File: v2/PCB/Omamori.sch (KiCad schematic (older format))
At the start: 28 parts, among them J1 Conn_01x04_Female, U1 BQ25504, U2 TPS61222DCK, U3 ATtiny85, U4 TS-1233

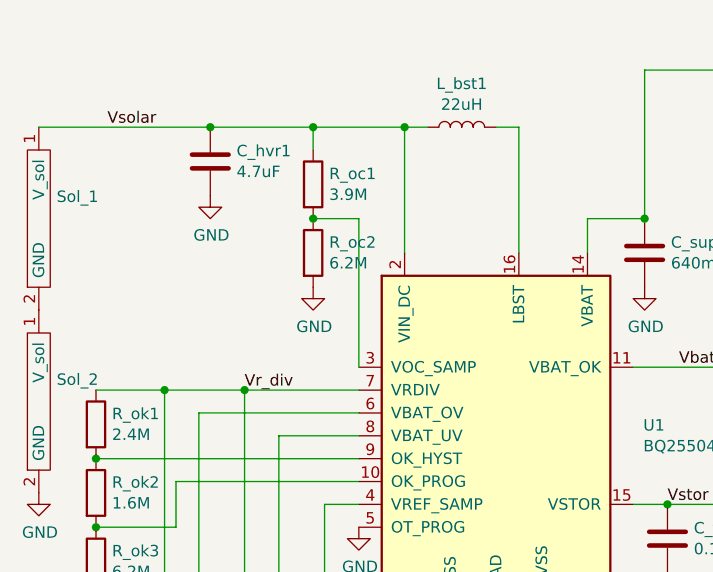
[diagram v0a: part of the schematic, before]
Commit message: Beyond last second changes to the PCB design and gerber files.
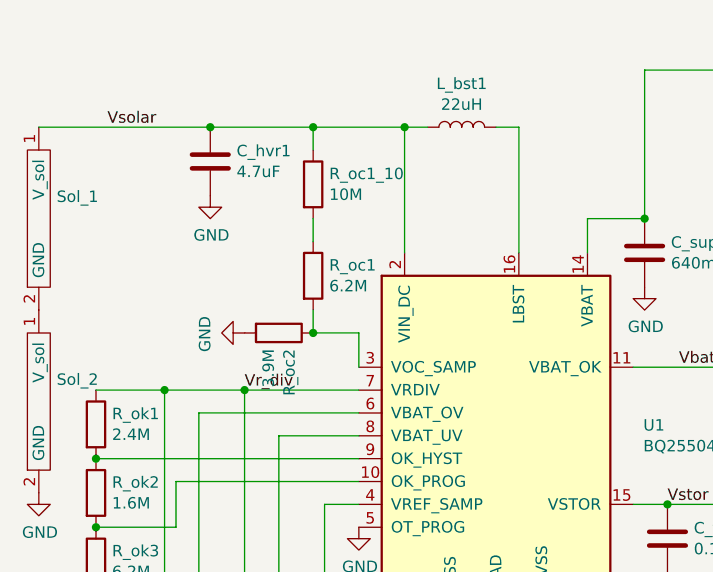
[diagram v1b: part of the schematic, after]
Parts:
- added R_oc1: 6.2M, Resistor_SMD:R_0603_1608Metric_Pad0.98x0.95mm_HandSolder, symbol Device:R
- R_oc1_10: renamed from R_oc1; value 3.9M -> 10M
- R_oc2: value 6.2M -> 3.9M
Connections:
- net at R_oc2.1, U1.3 (VOC_SAMP): now also R_oc1.2; no longer R_oc1_10.2
- new net: R_oc1.1, R_oc1_10.2
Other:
- moved on the sheet: R_oc2
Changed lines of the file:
@@
-$EndComp
-$Comp
-L Battery_Management:BQ25504 U1
-U 1 1 6049F0BD
-P 4550 3400
-F 0 "U1" H 5194 3446 50  0000 L CNN
-F 1 "BQ25504" H 5194 3355 50  0000 L CNN
-F 2 "footprints:VQFN-16-1EP_3x3mm_P0.5mm_EP1.8x1.8mm" H 4550 3400 50  0001 C CNN
-F 3 "http://www.ti.com/lit/ds/symlink/bq25504.pdf" H 4250 4200 50  0001 C CNN
-	1    4550 3400
-	1    0    0    -1
 $EndComp
 $Comp
@@
 Connection ~ 4150 2050
 $Comp
-L Device:R R_oc1
+L Device:R R_oc1_10
 U 1 1 609D50F7
 P 3750 2300
-F 0 "R_oc1" H 3820 2346 50  0000 L CNN
-F 1 "3.9M" H 3820 2255 50  0000 L CNN
+F 0 "R_oc1_10" H 3820 2346 50  0000 L CNN
+F 1 "10M" H 3820 2255 50  0000 L CNN
 F 2 "Resistor_SMD:R_0603_1608Metric_Pad1.05x0.95mm_HandSolder" V 3680 2300 50  0001 C CNN
 F 3 "~" H 3750 2300 50  0001 C CNN
@@
 L Device:R R_oc2
 U 1 1 609D577E
-P 3750 2600
-F 0 "R_oc2" H 3820 2646 50  0000 L CNN
-F 1 "6.2M" H 3820 2555 50  0000 L CNN
-F 2 "Resistor_SMD:R_0603_1608Metric_Pad1.05x0.95mm_HandSolder" V 3680 2600 50  0001 C CNN
-F 3 "~" H 3750 2600 50  0001 C CNN
-	1    3750 2600
-	1    0    0    -1
+P 3600 2950
+F 0 "R_oc2" H 3670 2996 50  0000 L CNN
+F 1 "3.9M" H 3670 2905 50  0000 L CNN
+F 2 "Resistor_SMD:R_0603_1608Metric_Pad1.05x0.95mm_HandSolder" V 3530 2950 50  0001 C CNN
+F 3 "~" H 3600 2950 50  0001 C CNN
+	1    3600 2950
+	0    1    1    0
 $EndComp
 Wire Wire Line
@@
 Wire Wire Line
 	3750 2050 4150 2050
-Wire Wire Line
-	3750 2450 3950 2450
-Wire Wire Line
-	3950 2450 3950 3100
-Connection ~ 3750 2450
 $Comp
 L power:GND #PWR06
 U 1 1 609DECA8
-P 3750 2750
-F 0 "#PWR06" H 3750 2500 50  0001 C CNN
-F 1 "GND" H 3755 2577 50  0000 C CNN
-F 2 "" H 3750 2750 50  0001 C CNN
-F 3 "" H 3750 2750 50  0001 C CNN
-	1    3750 2750
-	1    0    0    -1
+P 3450 2950
+F 0 "#PWR06" H 3450 2700 50  0001 C CNN
+F 1 "GND" H 3455 2777 50  0000 C CNN
+F 2 "" H 3450 2950 50  0001 C CNN
+F 3 "" H 3450 2950 50  0001 C CNN
+	1    3450 2950
+	0    1    1    0
 $EndComp
 Wire Wire Line
@@
 	5200 1800 5200 2450
 Connection ~ 5200 2450
+$Comp
+L Battery_Management:BQ25504 U1
+U 1 1 6049F0BD
+P 4550 3400
+F 0 "U1" H 5194 3446 50  0000 L CNN
+F 1 "BQ25504" H 5194 3355 50  0000 L CNN
+F 2 "footprints:VQFN-16-1EP_3x3mm_P0.5mm_EP1.8x1.8mm" H 4550 3400 50  0001 C CNN
+F 3 "http://www.ti.com/lit/ds/symlink/bq25504.pdf" H 4250 4200 50  0001 C CNN
+	1    4550 3400
+	1    0    0    -1
+$EndComp
+Wire Wire Line
+	3950 3100 3950 2950
+Wire Wire Line
+	3950 2950 3750 2950
+$Comp
+L Device:R R_oc1
+U 1 1 60AEA81A
+P 3750 2700
+F 0 "R_oc1" H 3820 2746 50  0000 L CNN
+F 1 "6.2M" H 3820 2655 50  0000 L CNN
+F 2 "Resistor_SMD:R_0603_1608Metric_Pad0.98x0.95mm_HandSolder" V 3680 2700 50  0001 C CNN
+F 3 "~" H 3750 2700 50  0001 C CNN
+	1    3750 2700
+	1    0    0    -1
+$EndComp
+Wire Wire Line
+	3750 2850 3750 2950
+Connection ~ 3750 2950
+Wire Wire Line
+	3750 2550 3750 2450
 $EndSCHEMATC
